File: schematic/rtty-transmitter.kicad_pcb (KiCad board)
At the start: 2 copper layers, 120 x 60 mm, 75 parts, among them J1 USB Type B Connector, J2 USBasp header, J3 2x5 Pin Header Connector Fema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, J4 Conn_01x02_Pin, J5 Conn_01x02_Pin, J6 Conn_01x02_Pin, J7 SMA Vertical Female, Q1 PN2222A, Q2 PN2222A, U1 MCP2221AxP, U2 ATmega328P-P, U3 MCP4901, U4 25LC1024, U5 MCP6022, Y1 16 MHz

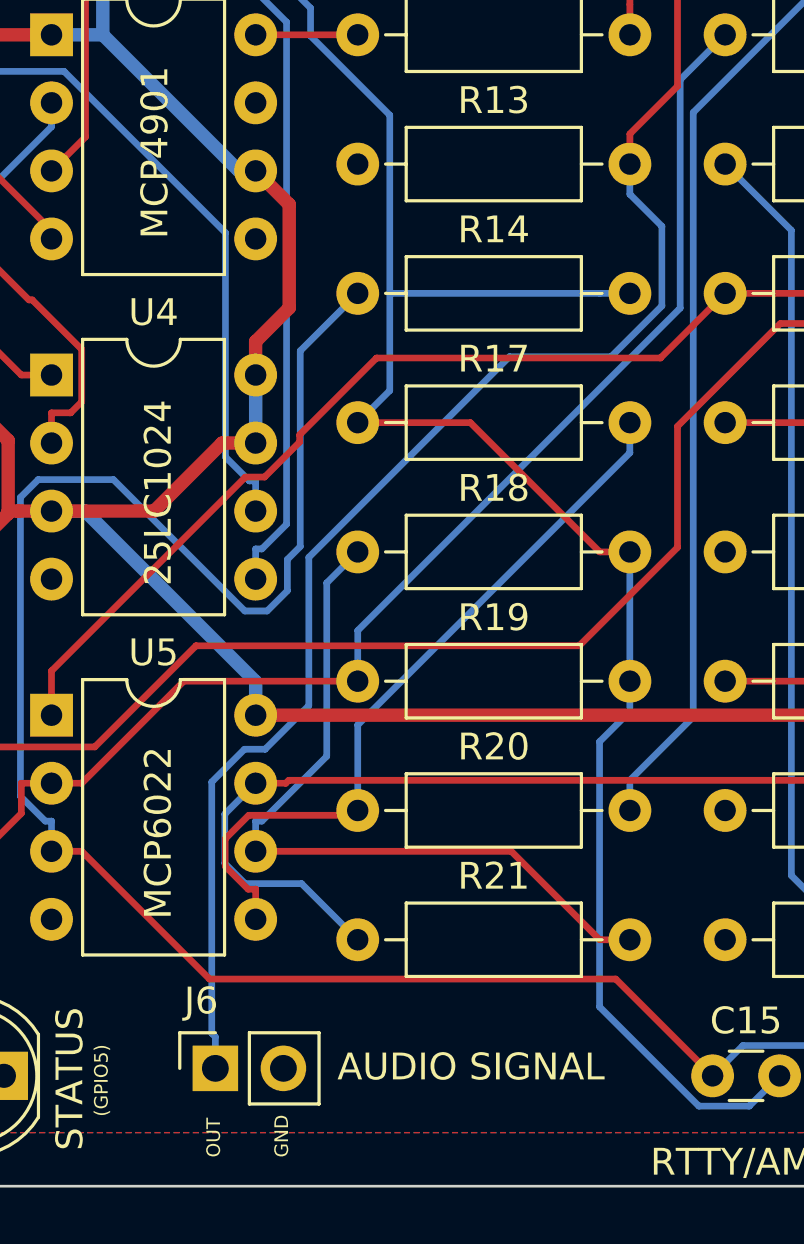
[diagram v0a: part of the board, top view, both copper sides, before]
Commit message: PCB: PCB layout updated
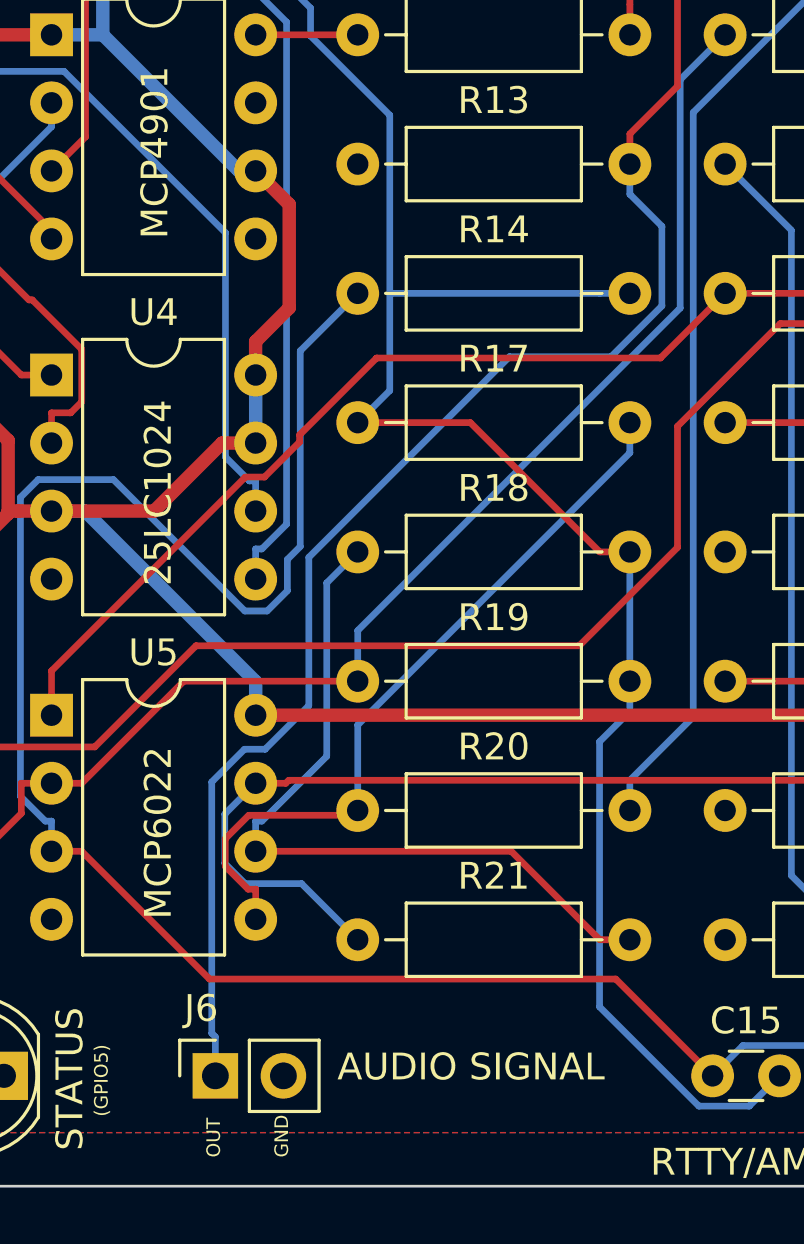
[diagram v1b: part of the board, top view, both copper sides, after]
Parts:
- moved J6 0.28 mm to (67.3, 55.9)
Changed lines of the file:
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@@
   )
   (footprint "Connector_PinSocket_2.54mm:PinSocket_1x02_P2.54mm_Vertical" (layer "F.Cu")
-    (at 67.33 55.601 90)
+    (at 67.33 55.88 90)
     (descr "Through hole straight socket strip, 1x02, 2.54mm pitch, single row (from Kicad 4.0.7), script generated")
     (tags "Through hole socket strip THT 1x02 2.54mm single row")
@@
   (segment (start 84.5821 10.8819) (end 84.5821 18.939) (width 0.25) (layer "F.Cu") (net 6))
   (segment (start 84.5821 18.939) (end 82.804 20.7171) (width 0.25) (layer "F.Cu") (net 6))
-  (segment (start 67.1955 54.2896) (end 67.1955 44.9112) (width 0.25) (layer "B.Cu") (net 6))
-  (segment (start 82.804 21.844) (end 82.804 22.9709) (width 0.25) (layer "B.Cu") (net 6))
+  (segment (start 78.3066 29.0353) (end 82.1056 29.0353) (width 0.25) (layer "B.Cu") (net 6))
+  (segment (start 82.804 22.9709) (end 82.804 21.844) (width 0.25) (layer "B.Cu") (net 6))
   (segment (start 88.606 6.858) (end 93.94 6.858) (width 0.25) (layer "B.Cu") (net 6))
   (segment (start 93.94 6.858) (end 95.464 8.382) (width 0.25) (layer "B.Cu") (net 6))
-  (segment (start 67.33 55.601) (end 67.33 54.4241) (width 0.25) (layer "B.Cu") (net 6))
-  (segment (start 78.3066 29.0353) (end 82.1056 29.0353) (width 0.25) (layer "B.Cu") (net 6))
-  (segment (start 84 24.1669) (end 82.804 22.9709) (width 0.25) (layer "B.Cu") (net 6))
-  (segment (start 87.082 8.382) (end 88.606 6.858) (width 0.25) (layer "B.Cu") (net 6))
-  (segment (start 84 27.1409) (end 84 24.1669) (width 0.25) (layer "B.Cu") (net 6))
-  (segment (start 69.1882 43.688) (end 70.8192 42.057) (width 0.25) (layer "B.Cu") (net 6))
-  (segment (start 70.8192 36.5227) (end 78.3066 29.0353) (width 0.25) (layer "B.Cu") (net 6))
-  (segment (start 70.8192 42.057) (end 70.8192 36.5227) (width 0.25) (layer "B.Cu") (net 6))
   (segment (start 82.1056 29.0353) (end 84 27.1409) (width 0.25) (layer "B.Cu") (net 6))
+  (segment (start 70.8192 42.057) (end 70.8192 36.5227) (width 0.25) (layer "B.Cu") (net 6))
+  (segment (start 67.1955 54.2896) (end 67.1955 44.9112) (width 0.25) (layer "B.Cu") (net 6))
   (segment (start 67.33 54.4241) (end 67.1955 54.2896) (width 0.25) (layer "B.Cu") (net 6))
   (segment (start 67.1955 44.9112) (end 68.4187 43.688) (width 0.25) (layer "B.Cu") (net 6))
+  (segment (start 87.082 8.382) (end 88.606 6.858) (width 0.25) (layer "B.Cu") (net 6))
+  (segment (start 67.33 55.88) (end 67.33 54.4241) (width 0.25) (layer "B.Cu") (net 6))
   (segment (start 68.4187 43.688) (end 69.1882 43.688) (width 0.25) (layer "B.Cu") (net 6))
+  (segment (start 70.8192 36.5227) (end 78.3066 29.0353) (width 0.25) (layer "B.Cu") (net 6))
+  (segment (start 69.1882 43.688) (end 70.8192 42.057) (width 0.25) (layer "B.Cu") (net 6))
+  (segment (start 84 27.1409) (end 84 24.1669) (width 0.25) (layer "B.Cu") (net 6))
+  (segment (start 84 24.1669) (end 82.804 22.9709) (width 0.25) (layer "B.Cu") (net 6))
   (segment (start 23.1724 47.853) (end 23.1724 39.1685) (width 0.25) (layer "F.Cu") (net 7))
   (segment (start 15.1454 55.88) (end 23.1724 47.853) (width 0.25) (layer "F.Cu") (net 7))
